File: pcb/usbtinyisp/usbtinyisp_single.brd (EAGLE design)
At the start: 44 x 36 mm, 20 parts, among them IC1 ATTINY2313-20P, IC2 74AHC125N

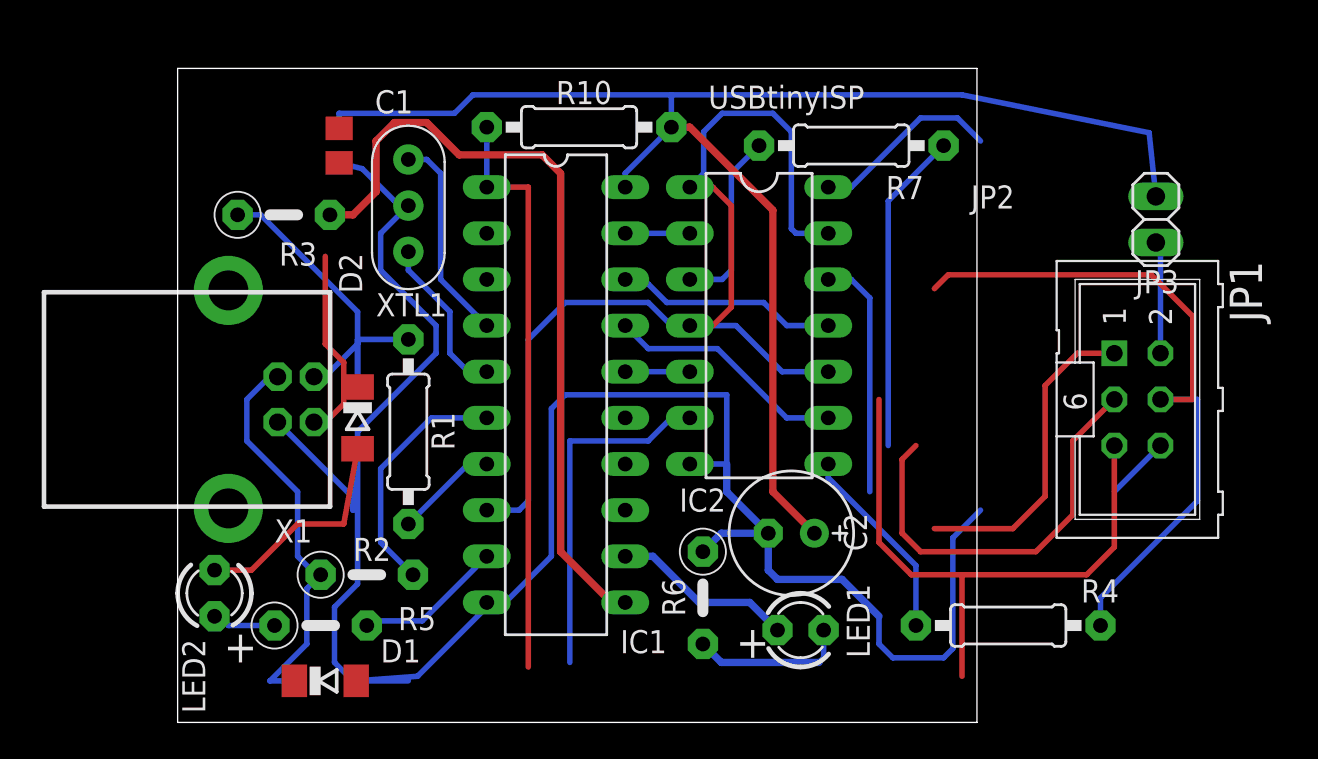
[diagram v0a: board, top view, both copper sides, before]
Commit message: unsmash
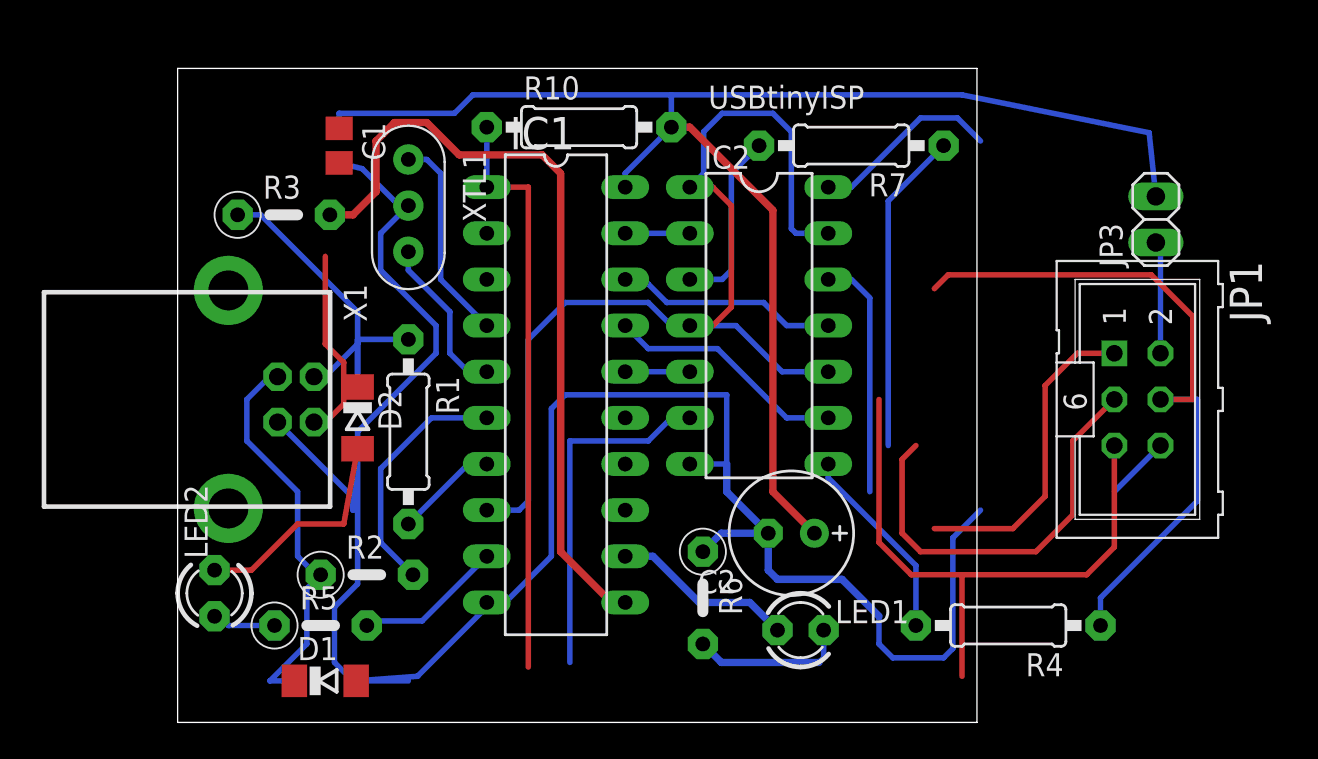
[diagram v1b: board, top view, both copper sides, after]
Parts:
- C1: value 0.1uF -> 100n
- C2: value 100uF -> 100u
- R10: value 10K -> 10k
- R3, R4, R5, R6, R7: value 1.5K -> 1k5
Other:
- board text removed: "+"
- board text removed: "C1"
- board text removed: "D1"
- board text removed: "D2"
- board text removed: "IC1"
- board text removed: "IC2"
- board text removed: "JP2"
- board text removed: "JP3"
- board text removed: "LED1"
- board text removed: "LED2"
- board text removed: "R1"
- board text removed: "R10"
- board text removed: "R2"
- board text removed: "R3"
- board text removed: "R4"
- board text removed: "R5"
- board text removed: "R6"
- board text removed: "R7"
- board text removed: "X1"
- board text removed: "XTL1"
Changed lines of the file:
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@@
 <setting verticaltext="up"/>
 </settings>
-<grid distance="100" unitdist="mil" unit="mil" style="lines" multiple="1" display="yes" altdistance="0.025" altunitdist="inch" altunit="mil"/>
+<grid distance="100" unitdist="mil" unit="mil" style="lines" multiple="1" display="no" altdistance="0.025" altunitdist="inch" altunit="mil"/>
 <layers>
 <layer number="1" name="Top" color="4" fill="1" visible="yes" active="yes"/>
@@
 <text x="6.096" y="29.718" size="1.016" layer="22" font="vector" rot="MR270">external</text>
 <text x="5.334" y="30.48" size="1.016" layer="22" font="vector" rot="MR90">power</text>
-<text x="5.588" y="25.146" size="1.27" layer="21" font="vector">R3</text>
-<text x="15.24" y="14.986" size="1.27" layer="21" font="vector" rot="R90">R1</text>
-<text x="12.954" y="34.798" size="1.27" layer="21" font="vector" rot="R180">C1</text>
-<text x="11.176" y="3.302" size="1.27" layer="21" font="vector">D1</text>
-<text x="10.16" y="23.622" size="1.27" layer="21" font="vector" rot="R90">D2</text>
-<text x="10.922" y="22.352" size="1.27" layer="21" font="vector">XTL1</text>
-<text x="5.334" y="9.906" size="1.27" layer="21" font="vector">X1</text>
-<text x="36.83" y="7.62" size="1.27" layer="21" font="vector" rot="R270">LED1</text>
-<text x="1.524" y="0.508" size="1.27" layer="21" font="vector" rot="R90">LED2</text>
-<text x="51.816" y="7.874" size="1.27" layer="21" font="vector" rot="R180">R4</text>
-<text x="14.224" y="6.35" size="1.27" layer="21" font="vector" rot="R180">R5</text>
-<text x="27.94" y="5.842" size="1.27" layer="21" font="vector" rot="R90">R6</text>
-<text x="38.9865" y="28.8061" size="1.27" layer="21" font="vector">R7</text>
-<text x="20.828" y="34.036" size="1.27" layer="21" font="vector">R10</text>
-<text x="9.652" y="8.89" size="1.27" layer="21" font="vector">R2</text>
-<text x="46.068" y="29.558" size="1.27" layer="21" font="vector" rot="R180">JP2</text>
-<text x="55.118" y="24.892" size="1.27" layer="21" font="vector" rot="R180">JP3</text>
-<text x="26.924" y="5.08" size="1.27" layer="21" font="vector" rot="R180">IC1</text>
 <text x="21.59" y="9.906" size="1.27" layer="22" font="vector" rot="MR90">www.ladyada.net/</text>
 <text x="19.558" y="11.684" size="1.27" layer="22" font="vector" rot="MR90">make/usbtiny</text>
 <text x="29.21" y="33.782" size="1.27" layer="21" font="vector">USBtinyISP</text>
-<text x="30.734" y="3.556" size="1.778" layer="21" font="vector">+</text>
-<text x="27.61741875" y="11.60271875" size="1.27" layer="21" font="vector">IC2</text>
-<text x="2.54" y="3.302" size="1.778" layer="21" font="vector">+</text>
 </plain>
 <attributes>
@@
 </autorouter>
 <elements>
-<element name="R1" library="rcl-ez" package="0207/10" value="68" x="12.7" y="16.002" smashed="yes" rot="R270">
-<attribute name="VALUE" x="14.605" y="20.2946" size="1.27" layer="27" ratio="10" rot="R270"/>
-</element>
-<element name="R2" library="rcl-ez" package="0207/5V" value="68" x="10.414" y="8.128" smashed="yes">
-<attribute name="VALUE" x="4.5466" y="9.525" size="1.27" layer="27" ratio="10" rot="R180"/>
-</element>
-<element name="R3" library="rcl-ez" package="0207/5V" value="1.5K" x="5.842" y="27.94" smashed="yes">
-<attribute name="VALUE" x="3.8354" y="27.305" size="1.27" layer="27" ratio="10"/>
-</element>
-<element name="XTL1" library="minimidi" package="CERM_OSC" value="12.0 MHz" x="12.7" y="28.448" smashed="yes" rot="R270">
-<attribute name="VALUE" x="10.486" y="31.948" size="1.27" layer="27" rot="R270"/>
-</element>
-<element name="IC1" library="avr" package="DIL20" value="ATTINY2313-20P" x="20.828" y="18.034" smashed="yes" rot="R270">
-<attribute name="VALUE" x="20.066" y="28.194" size="1.778" layer="27" ratio="10" rot="R270"/>
-</element>
-<element name="JP3" library="pinhead" package="1X02" value="PWR" x="53.848" y="27.686" smashed="yes" rot="R90">
-<attribute name="VALUE" x="57.023" y="25.146" size="1.27" layer="27" rot="R90"/>
-</element>
-<element name="C1" library="rcl" package="C0805" value="0.1uF" x="8.89" y="31.75" smashed="yes" rot="R270">
-<attribute name="VALUE" x="10.668" y="33.528" size="1.27" layer="27" ratio="10" rot="R270"/>
-</element>
-<element name="LED1" library="minimidi" package="LED3MM" value="" x="34.29" y="5.08" smashed="yes">
-<attribute name="VALUE" x="36.195" y="3.429" size="1.27" layer="27" ratio="10"/>
-</element>
-<element name="R6" library="rcl-ez" package="0207/5V" value="1.5K" x="28.9123" y="6.858" smashed="yes" rot="R270">
-<attribute name="VALUE" x="28.2773" y="9.1186" size="1.27" layer="27" ratio="10" rot="R270"/>
-</element>
-<element name="D1" library="diode" package="SOD80C" value="3V6" x="8.128" y="2.286" smashed="yes">
-<attribute name="VALUE" x="1.524" y="1.27" size="1.27" layer="27" ratio="10" rot="R90"/>
-</element>
-<element name="D2" library="diode" package="SOD80C" value="3V6" x="9.906" y="16.764" smashed="yes" rot="R270">
-<attribute name="VALUE" x="5.588" y="10.414" size="1.27" layer="27" ratio="10"/>
-</element>
-<element name="R7" library="rcl-ez" package="0207/10" value="1.5K" x="37.084" y="31.75" smashed="yes" rot="R180">
-<attribute name="VALUE" x="41.275" y="32.639" size="1.27" layer="27" ratio="10" rot="R270"/>
-</element>
-<element name="R4" library="rcl-ez" package="0207/10" value="1.5K" x="45.72" y="5.334" smashed="yes" rot="R180">
-<attribute name="VALUE" x="46.863" y="7.493" size="1.27" layer="27" ratio="10" rot="R180"/>
-</element>
-<element name="R10" library="rcl-ez" package="0207/10" value="10K" x="22.098" y="32.766" smashed="yes">
-<attribute name="VALUE" x="20.955" y="30.607" size="1.27" layer="27" ratio="10"/>
-</element>
-<element name="R5" library="rcl-ez" package="0207/5V" value="1.5K" x="7.874" y="5.334" smashed="yes">
-<attribute name="VALUE" x="5.6134" y="4.699" size="1.27" layer="27" ratio="10"/>
-</element>
-<element name="LED2" library="minimidi" package="LED3MM" value="" x="2.032" y="7.112" smashed="yes" rot="R90">
-<attribute name="VALUE" x="3.683" y="9.017" size="1.27" layer="27" ratio="10" rot="R90"/>
-</element>
+<element name="R1" library="rcl-ez" package="0207/10" value="68" x="12.7" y="16.002" rot="R270"/>
+<element name="R2" library="rcl-ez" package="0207/5V" value="68" x="10.414" y="8.128"/>
+<element name="R3" library="rcl-ez" package="0207/5V" value="1k5" x="5.842" y="27.94"/>
+<element name="XTL1" library="minimidi" package="CERM_OSC" value="12.0 MHz" x="12.7" y="28.448" rot="R270"/>
+<element name="IC1" library="avr" package="DIL20" value="ATTINY2313-20P" x="20.828" y="18.034" rot="R270"/>
+<element name="JP3" library="pinhead" package="1X02" value="PWR" x="53.848" y="27.686" rot="R90"/>
+<element name="C1" library="rcl" package="C0805" value="100n" x="8.89" y="31.75" rot="R270"/>
+<element name="LED1" library="minimidi" package="LED3MM" value="" x="34.29" y="5.08"/>
+<element name="R6" library="rcl-ez" package="0207/5V" value="1k5" x="28.9123" y="6.858" rot="R270"/>
+<element name="D1" library="diode" package="SOD80C" value="3V6" x="8.128" y="2.286"/>
+<element name="D2" library="diode" package="SOD80C" value="3V6" x="9.906" y="16.764" rot="R270"/>
+<element name="R7" library="rcl-ez" package="0207/10" value="1k5" x="37.084" y="31.75" rot="R180"/>
+<element name="R4" library="rcl-ez" package="0207/10" value="1k5" x="45.72" y="5.334" rot="R180"/>
+<element name="R10" library="rcl-ez" package="0207/10" value="10k" x="22.098" y="32.766"/>
+<element name="R5" library="rcl-ez" package="0207/5V" value="1k5" x="7.874" y="5.334"/>
+<element name="LED2" library="minimidi" package="LED3MM" value="" x="2.032" y="7.112" rot="R90"/>
 <element name="JP1" library="con-ml" package="ML6" value="" x="52.832" y="17.78" rot="R270">
 <attribute name="OC_NEWARK" value="unknown" x="52.832" y="17.78" size="1.778" layer="27" rot="R270" display="off"/>
@@
 <attribute name="OC_FARNELL" value="unknown" x="52.832" y="17.78" size="1.778" layer="27" rot="R270" display="off"/>
 </element>
-<element name="X1" library="con-berg-ez" package="PN61729" value="" x="2.794" y="17.78" smashed="yes" rot="R270">
-<attribute name="VALUE" x="-6.096" y="10.16" size="1.27" layer="27"/>
-</element>
-<element name="IC2" library="74xx-eu" package="DIL14" value="74AHC125N" x="32.004" y="21.844" smashed="yes" rot="R270">
-<attribute name="VALUE" x="31.369" y="28.575" size="1.27" layer="27" ratio="10" rot="R270"/>
-</element>
-<element name="C2" library="rcl" package="E2,5-7" value="100uF" x="33.782" y="10.414" smashed="yes" rot="R180">
-<attribute name="NAME" x="36.675" y="11.5189" size="1.27" layer="25" font="vector" ratio="10" rot="R270"/>
-<attribute name="VALUE" x="31.369" y="12.827" size="1.27" layer="27" ratio="10" rot="R180"/>
-</element>
+<element name="X1" library="con-berg-ez" package="PN61729" value="" x="2.794" y="17.78" rot="R270"/>
+<element name="IC2" library="74xx-eu" package="DIL14" value="74AHC125N" x="32.004" y="21.844" rot="R270"/>
+<element name="C2" library="rcl" package="E2,5-7" value="100u" x="33.782" y="10.414" rot="R180"/>
 </elements>
 <signals>
@@
 <wire x1="28.194" y1="32.766" x2="32.766" y2="28.194" width="0.4064" layer="1"/>
 <wire x1="27.178" y1="32.766" x2="28.194" y2="32.766" width="0.4064" layer="1"/>
+<wire x1="8.89" y1="32.7" x2="8.89" y2="32.7" width="0" layer="19" extent="1-16"/>
 <wire x1="8.128" y1="25.654" x2="8.89" y2="32.7" width="0" layer="19" extent="1-1"/>
 </signal>

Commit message: vergessene Änderungen
wenn man nicht alles gleich commited :-/
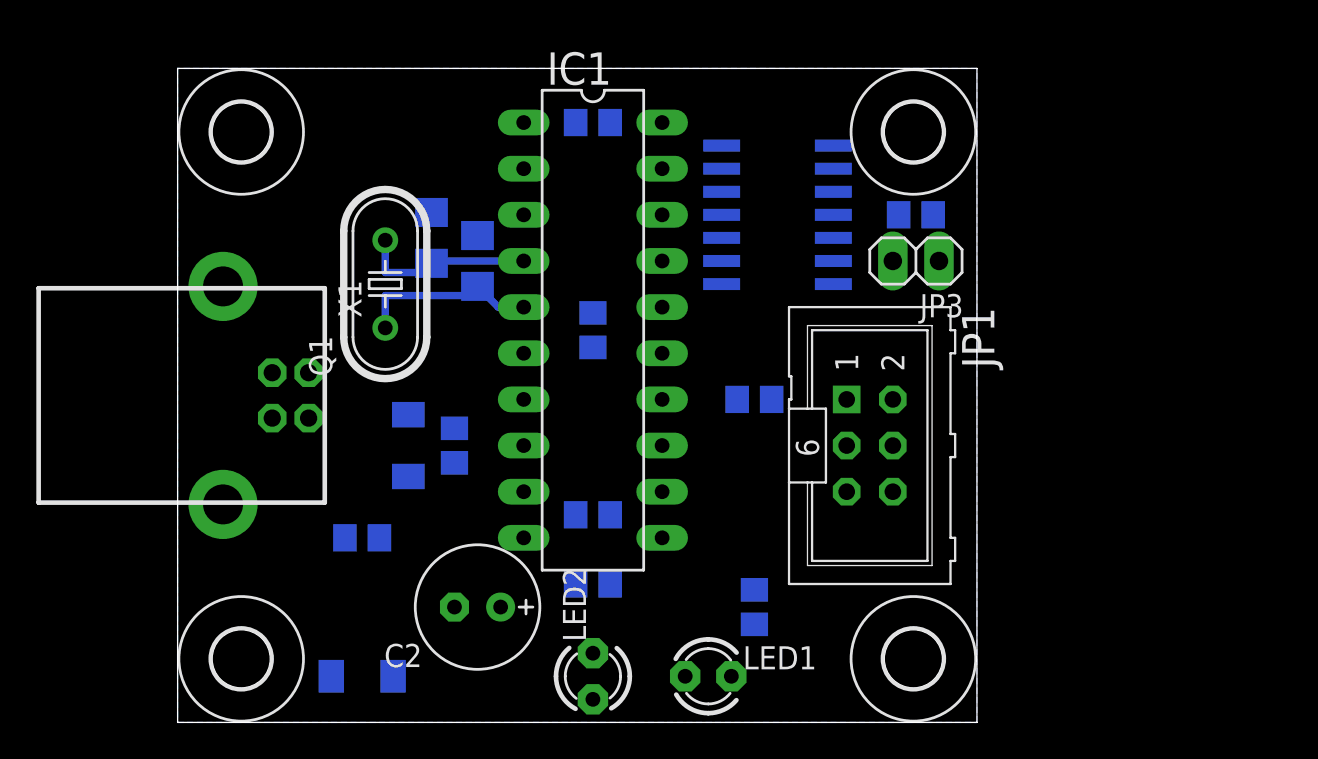
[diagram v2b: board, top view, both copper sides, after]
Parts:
- removed XTL1: 12.0 MHz, minimidi:CERM_OSC
- added C3, C4: 22p, rcl:C1206
- added Q1: 12000, crystal:HC49U-V
- added U$1, U$2, U$3, U$4: (no value), holes:3,2
- IC2: value 74AHC125N -> 74LVX125D; device 74xx-eu:DIL14 -> 74xx-eu:SO14
- R1, R10, R4, R7: device rcl-ez:0207/10 -> rcl:R0805
- R2, R3, R5, R6: device rcl-ez:0207/5V -> rcl:R0805
- moved R3 26.5 mm to (22.9, 7.62), flipped to the bottom, turned to 180 degrees
- moved LED2 21.3 mm to (22.9, 2.54)
- moved R4 18.7 mm to (31.8, 17.8), flipped to the bottom, turned to 0 degrees
- moved C2 17.7 mm to (16.5, 6.35)
- moved C1 17.3 mm to (22.9, 21.6), flipped to the bottom
- moved R5 16.2 mm to (22.9, 11.4), flipped to the bottom, turned to 180 degrees
- moved JP1 14.9 mm to (38.1, 15.2)
- moved JP3 13.4 mm to (40.6, 25.4), turned to 180 degrees
- moved IC2 6.18 mm to (33.0, 27.9), flipped to the bottom
- moved LED1 5.68 mm to (29.2, 2.54)
- moved R7 5.21 mm to (40.6, 27.9), flipped to the bottom, turned to 0 degrees
- moved IC1 4.10 mm to (22.9, 21.6)
- moved D2 3.18 mm to (12.7, 15.2), flipped to the bottom
- moved R6 2.88 mm to (31.8, 6.35), flipped to the bottom
- moved R1 2.65 mm to (15.2, 15.2), flipped to the bottom
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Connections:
- removed net N$4: IC1.5, XTL1.P$3
- removed net N$5: IC1.4, XTL1.P$1
- new net XTAL1: C4.1, IC1.5, Q1.1
- new net XTAL2: C3.1, IC1.4, Q1.2
- net GND: now also C3.2, C4.2; no longer XTL1.P$2
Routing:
- net GND: track 134.5 -> 0.00 mm
- net VCC: track 92.5 -> 0.00 mm
- net N$15: track 58.3 -> 0.00 mm
- net RST: track 52.7 -> 0.00 mm
- net N$16: track 43.4 -> 0.00 mm
- net SCK: track 40.9 -> 0.00 mm
- net MOSI: track 38.5 -> 0.00 mm
- net N$9: track 32.0 -> 0.00 mm
- net MISO: track 30.8 -> 0.00 mm
- net N$2: track 22.0 -> 0.00 mm
- net N$1: track 21.8 -> 0.00 mm
- net N$14: track 17.1 -> 0.00 mm
- net N$6: track 13.6 -> 0.00 mm
- net MOSI': track 13.5 -> 0.00 mm
- net MISO': track 12.2 -> 0.00 mm
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- added copper zone on layer 16, net GND
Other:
- board text removed: "AVR"
- board text removed: "Dongle"
- board text removed: "GND"
- board text removed: "MISO"
- board text removed: "MOSI"
- board text removed: "N/C"
- board text removed: "RST"
- board text removed: "SCK"
- board text removed: "SpokePOV"
- board text removed: "USB"
- board text removed: "USBtiny"
- board text removed: "USBtinyISP"
- board text removed: "VCC"
- board text removed: "cut to use"
- board text removed: "external"
- board text removed: "make/usbtiny"
- board text removed: "power"
- board text removed: "programmer"
- board text removed: "www.ladyada.net/"
